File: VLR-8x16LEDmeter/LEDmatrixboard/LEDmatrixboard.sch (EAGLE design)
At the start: 20 parts, among them IC1 74HC595, IC2 74HC595, IC3 74HC595

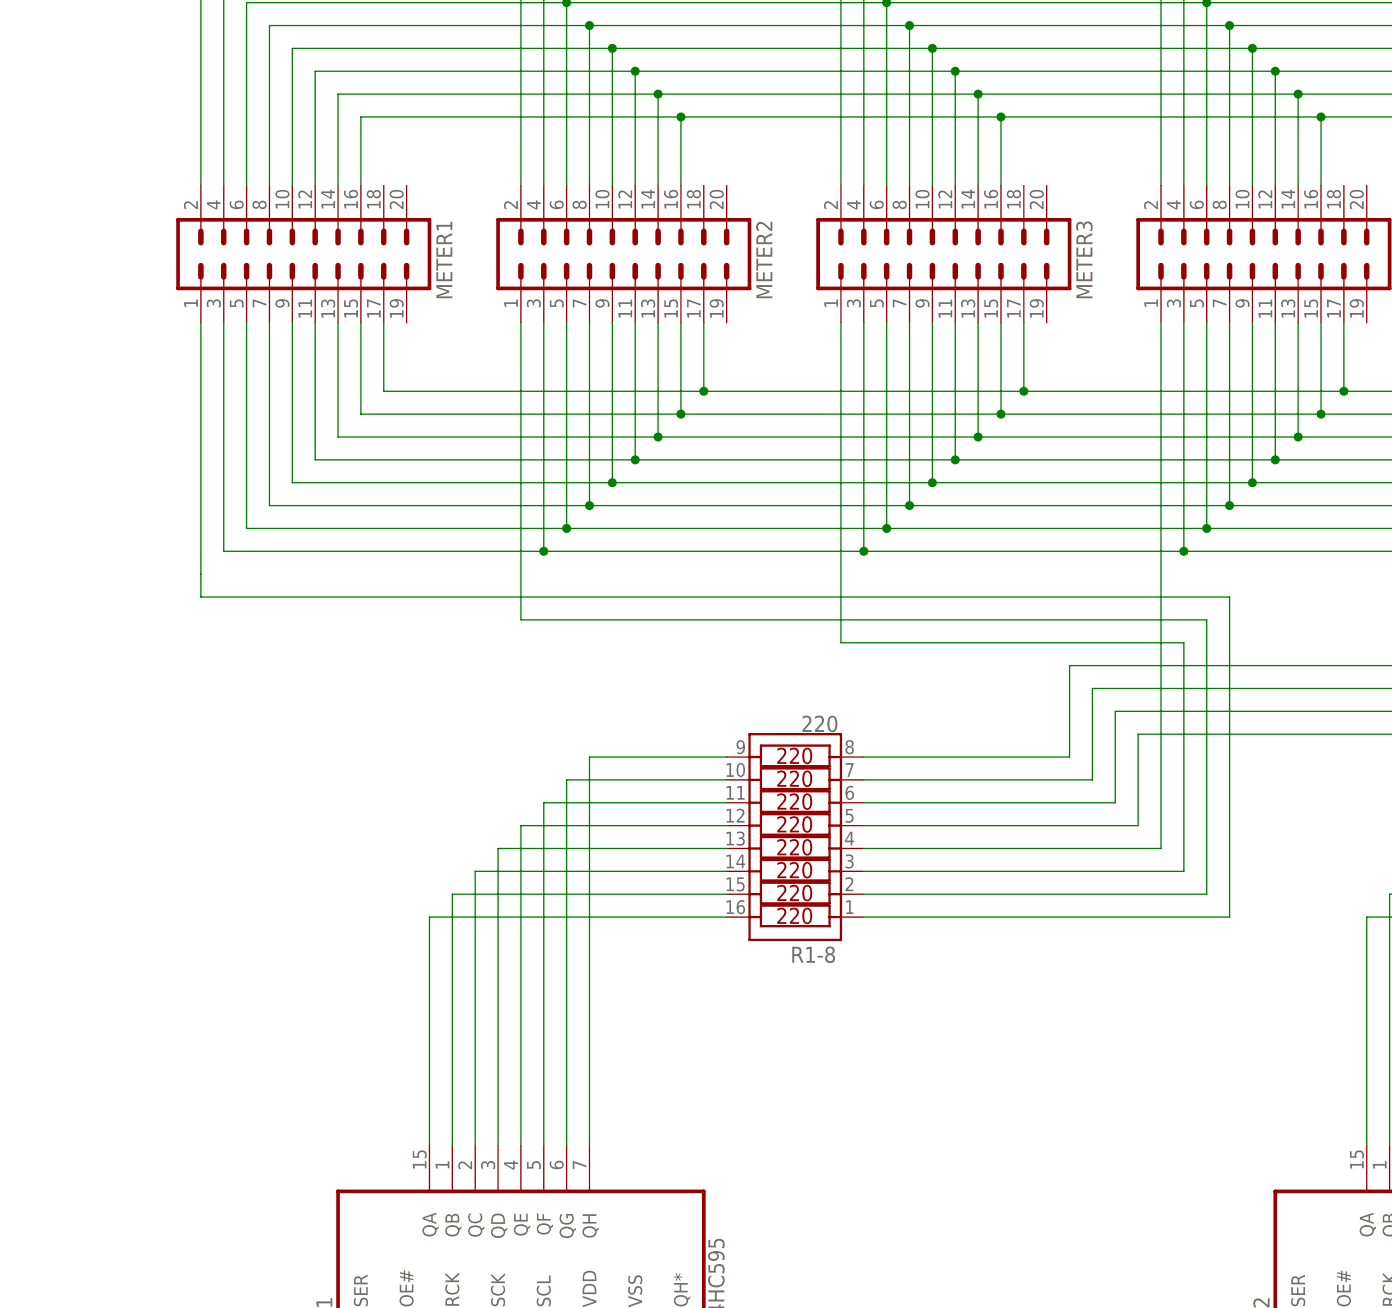
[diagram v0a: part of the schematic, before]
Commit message: update LEDMatrixboardV2.2.1
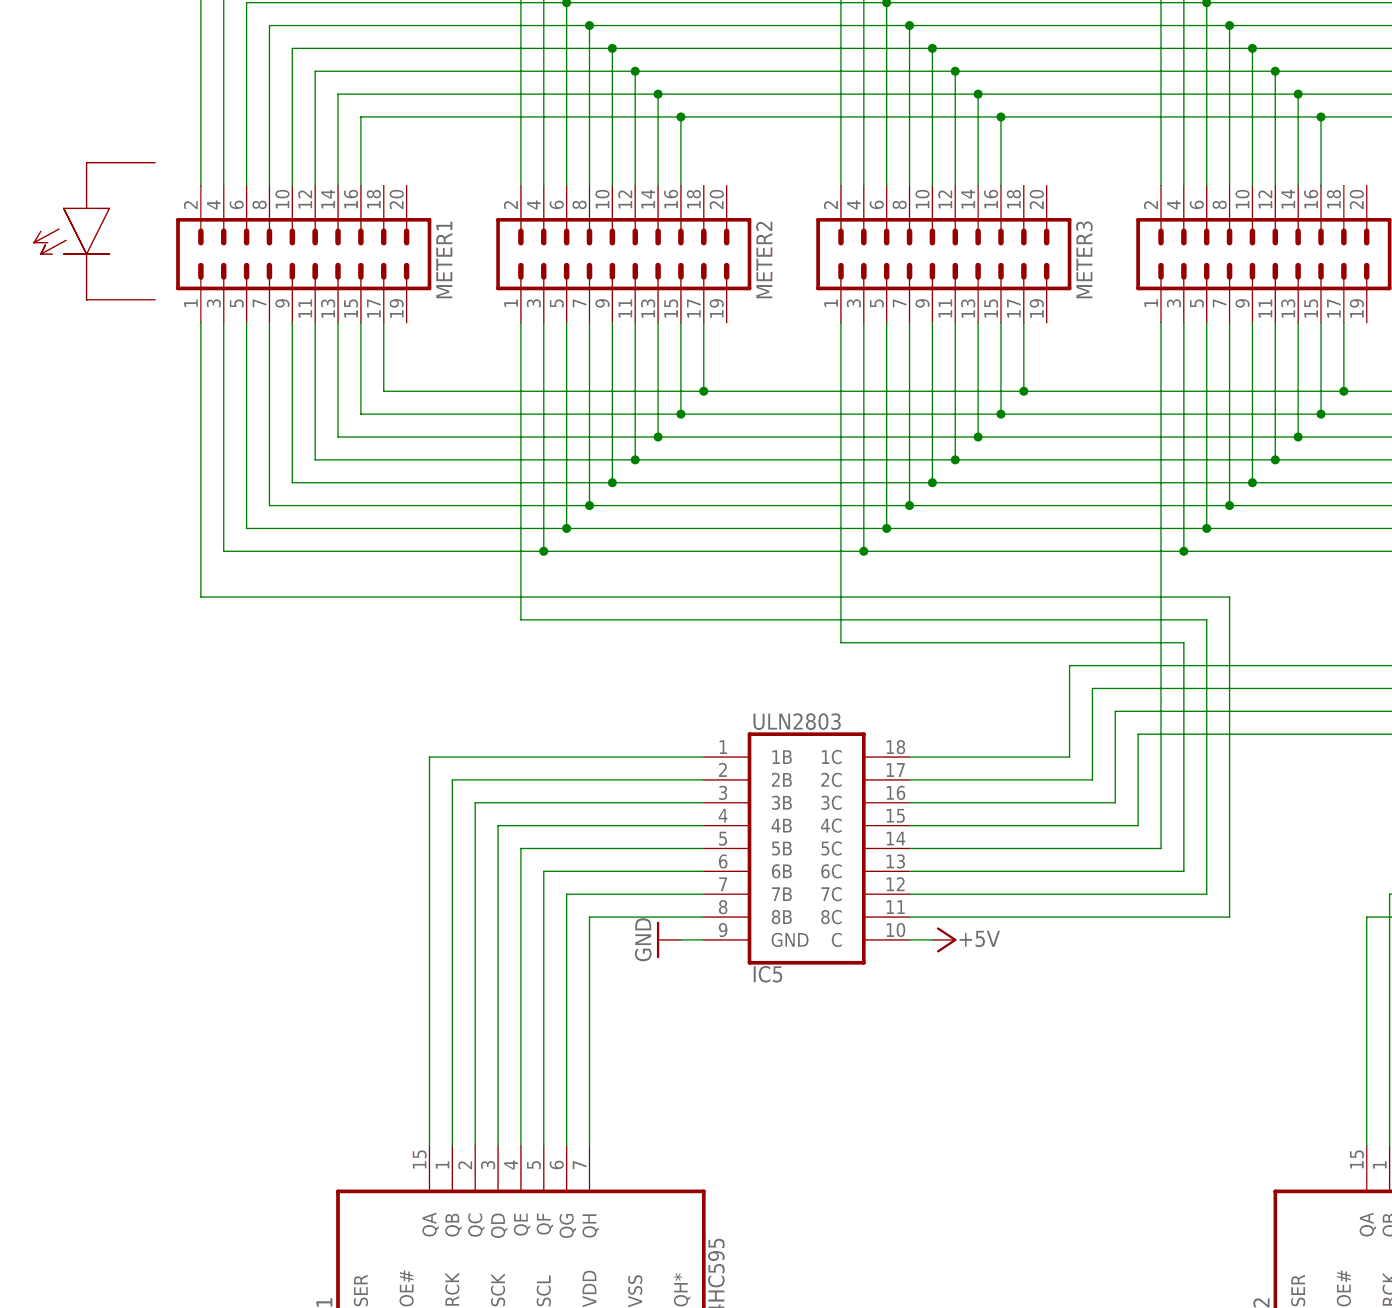
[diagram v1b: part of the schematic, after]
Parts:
- removed R1-8: 220, Bourns Resistor Array:4816P-1SOIC16W
- added IC5: ULN2803, 595-541-165-uln2803:ULN2803SO18W
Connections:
- net +5V: now also IC5.C
- net GND: now also IC5.GND
- net N$1: now also IC1.QH, IC5.8B; no longer IC1.QA, R1-8.P$16
- net N$34: now also IC1.QG, IC5.7B; no longer IC1.QB, R1-8.P$15
- net N$35: now also IC1.QF, IC5.6B; no longer IC1.QC, R1-8.P$14
- net N$36: now also IC1.QE, IC5.5B; no longer IC1.QD, R1-8.P$13
- net N$37: now also IC1.QD, IC5.4B; no longer IC1.QE, R1-8.P$12
- net N$38: now also IC1.QC, IC5.3B; no longer IC1.QF, R1-8.P$11
- net N$39: now also IC1.QB, IC5.2B; no longer IC1.QG, R1-8.P$10
- net N$40: now also IC1.QA, IC5.1B; no longer IC1.QH, R1-8.P$9
- net N$41: now also IC5.8C; no longer R1-8.P$1
- net N$42: now also IC5.7C; no longer R1-8.P$2
- net N$43: now also IC5.6C; no longer R1-8.P$3
- net N$44: now also IC5.5C; no longer R1-8.P$4
- net N$45: now also IC5.4C; no longer R1-8.P$5
- net N$46: now also IC5.3C; no longer R1-8.P$6
- net N$47: now also IC5.2C; no longer R1-8.P$7
- net N$48: now also IC5.1C; no longer R1-8.P$8
